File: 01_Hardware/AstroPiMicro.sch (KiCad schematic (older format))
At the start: 40 parts, among them J1 RPi Connector, J10 6-pin JST PH, J2 USB_C_Receptacle_USB2.0, J3 2-pin JST PH, J4 4-pin JST SH, J5 4-pin JST SH, J6 11-pin JST PH, J7 3-pin JST PH, J8 3-pin JST PH, J9 6-pin JST PH, SW1 SW-ON-OFF, U1 LM809, U2 STM32G431KBTx, U3 MCP73831-2-OT, U4 TPS61090, U5 Joystick, Y1 16MHz

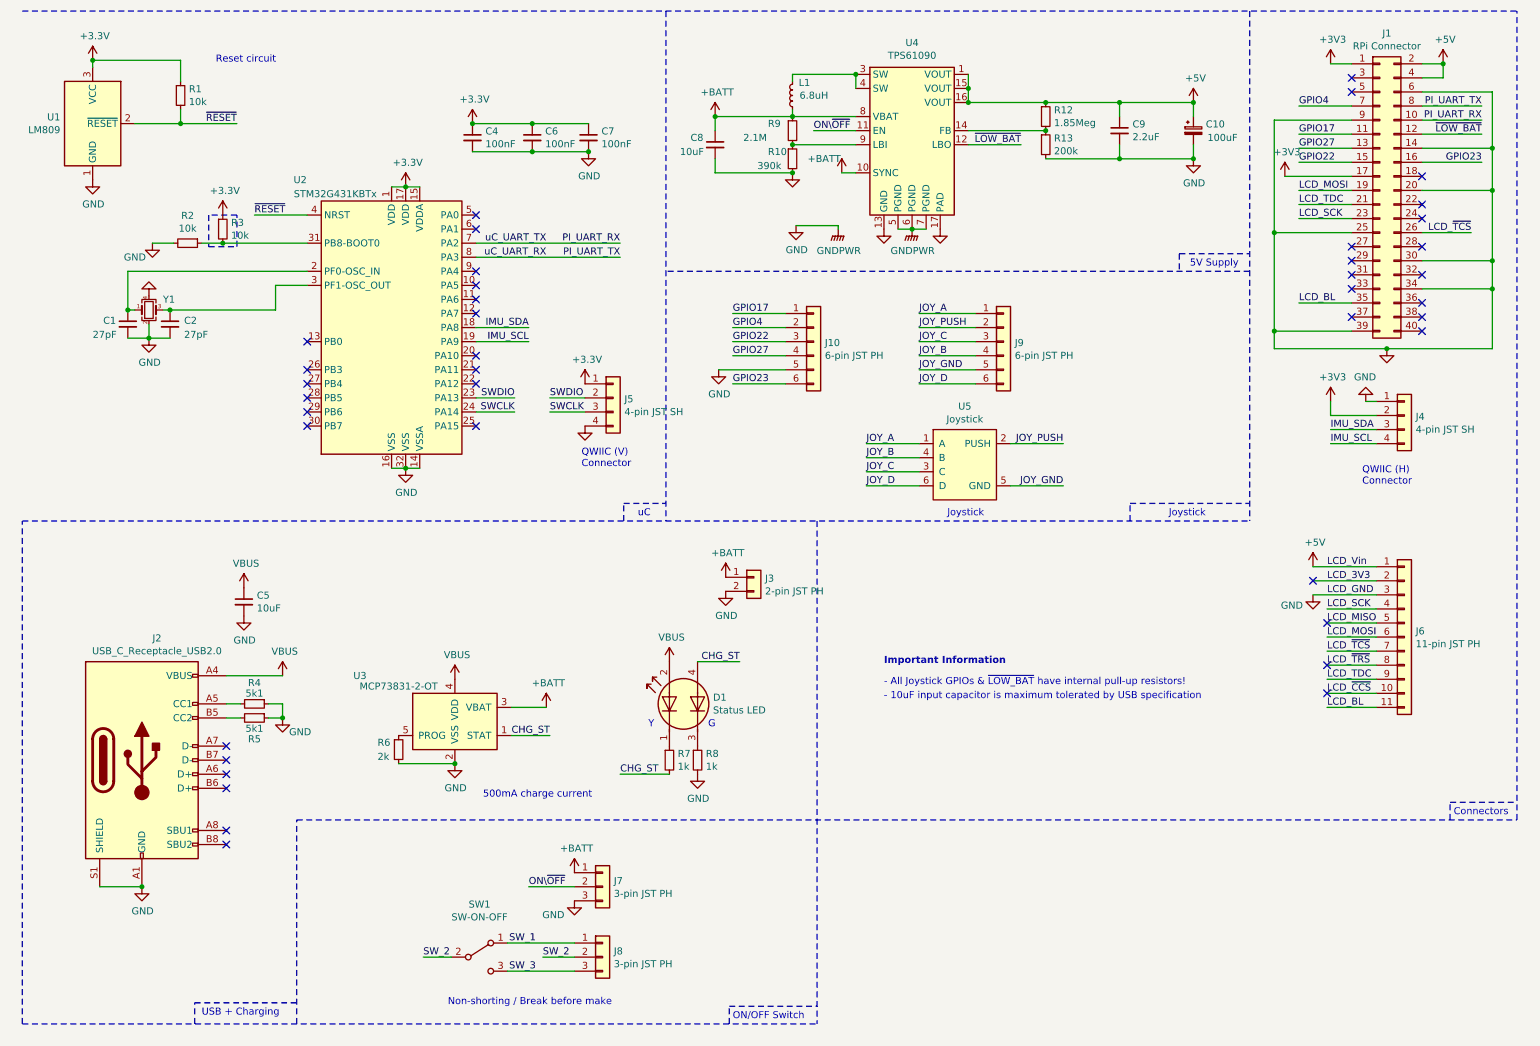
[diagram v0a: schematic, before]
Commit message: Started on HW version 2
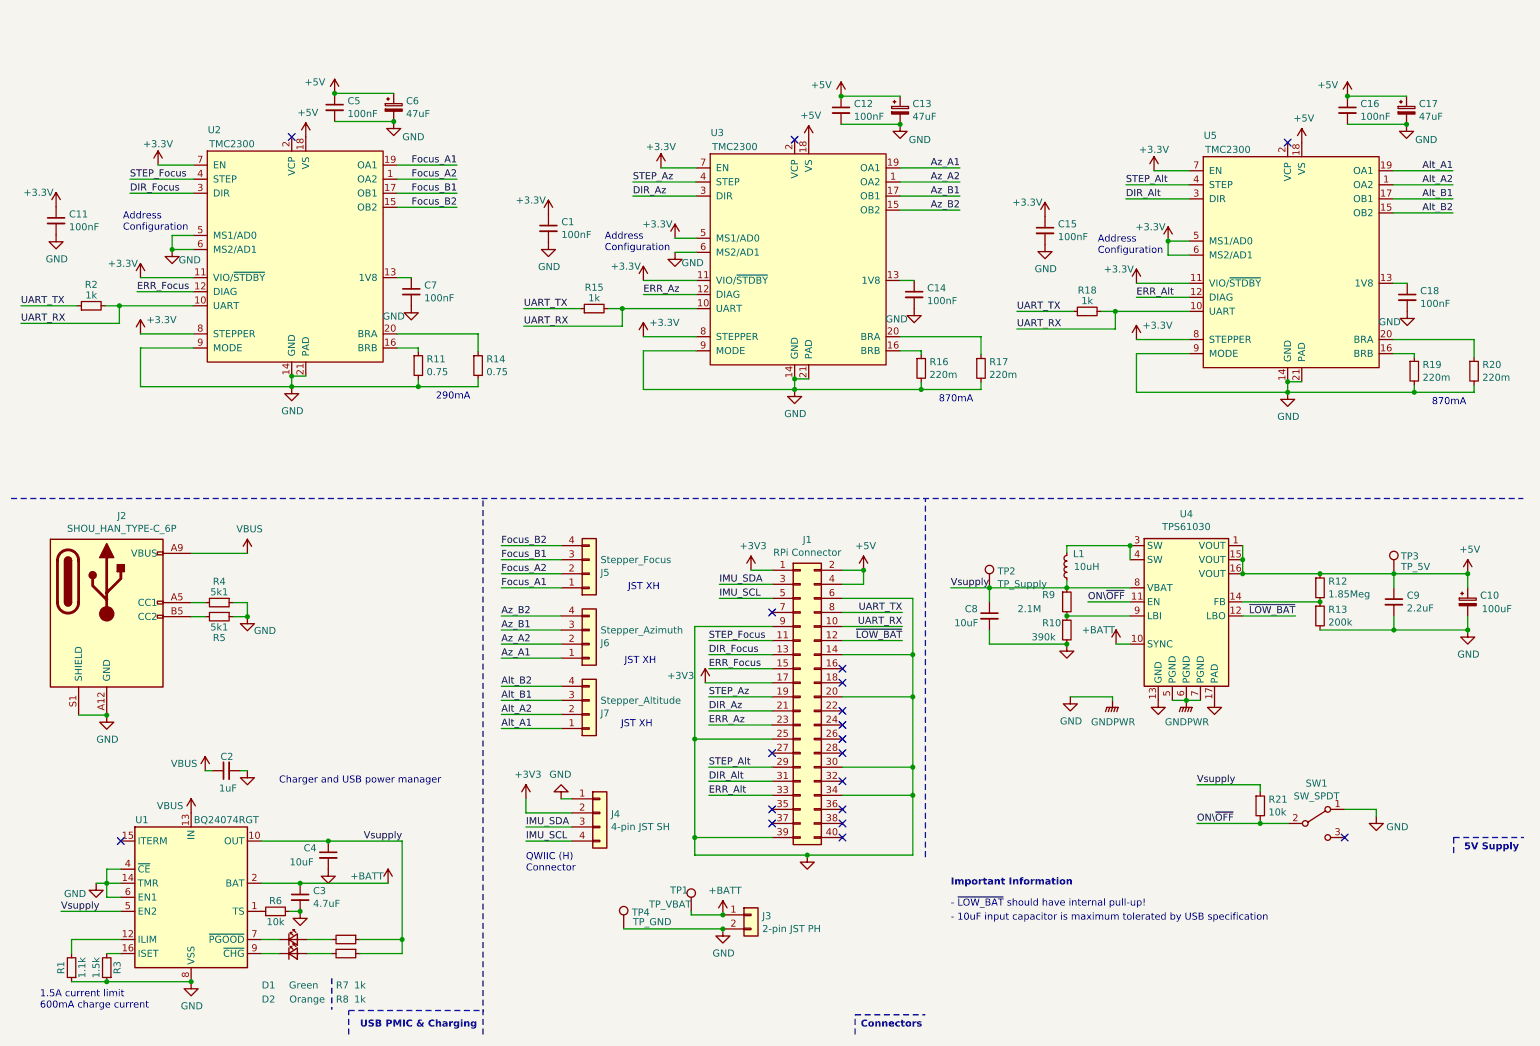
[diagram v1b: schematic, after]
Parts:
- removed C6: 100nF, Capacitor_SMD:C_0603_1608Metric_Pad1.05x0.95mm_HandSolder, symbol Device:C_Small
- removed D1: Status LED, LED_SMD:LED_Avago_PLCC4_3.2x2.8mm_CW, symbol Device:LED_Dual_CACA
- removed J10: 6-pin JST PH, Connector_JST:JST_PH_B6B-PH-K_1x06_P2.00mm_Vertical, symbol Connector_Generic:Conn_01x06
- removed J2: USB_C_Receptacle_USB2.0, astropi:USB_C_GCT_USB4085, symbol Connector:USB_C_Receptacle_USB2.0
- removed J6: 11-pin JST PH, Connector_JST:JST_PH_B11B-PH-K_1x11_P2.00mm_Vertical, symbol Connector_Generic:Conn_01x11
- removed J7: 3-pin JST PH, Connector_JST:JST_PH_B3B-PH-K_1x03_P2.00mm_Vertical, symbol Connector_Generic:Conn_01x03
- removed J8: 3-pin JST PH, Connector_JST:JST_PH_B3B-PH-SM4-TB_1x03-1MP_P2.00mm_Vertical, symbol Connector_Generic:Conn_01x03
- removed J9: 6-pin JST PH, Connector_JST:JST_PH_B6B-PH-SM4-TB_1x06-1MP_P2.00mm_Vertical, symbol Connector_Generic:Conn_01x06
- removed U1: LM809, Package_TO_SOT_SMD:SOT-23, symbol Power_Supervisor:LM809
- removed U2: STM32G431KBTx, Package_QFP:LQFP-32_7x7mm_P0.8mm, symbol MCU_ST_STM32G4:STM32G431KBTx
- removed U3: MCP73831-2-OT, Package_TO_SOT_SMD:SOT-23-5, symbol Battery_Management:MCP73831-2-OT
- removed U5: Joystick, astropi:SKRHAAE010, symbol joystick:SKRHAAE010
- removed Y1: 16MHz, Crystal:Crystal_SMD_Abracon_ABM3B-4Pin_5.0x3.2mm, symbol Device:Crystal_GND24_Small
- added C11, C12, C14, C15, C16, C18: 100nF, Capacitor_SMD:C_0603_1608Metric, symbol Device:C_Small
- added C13, C17, C6: 47uF, Capacitor_Tantalum_SMD:CP_EIA-3528-15_AVX-H, symbol Device:CP_Small
- added C3: 4.7uF, Capacitor_SMD:C_0805_2012Metric, symbol Device:C_Small
- added D1: Green, LED_SMD:LED_0603_1608Metric, symbol Device:LED_Small
- added D2: Orange, LED_SMD:LED_0603_1608Metric, symbol Device:LED_Small
- added J2: SHOU_HAN_TYPE-C_6P, astropi:SHOU HAN TYPE-C 6P, symbol astropi:SHOU_HAN_TYPE-C_6P
- added J6: Stepper_Azimuth, Connector_JST:JST_XH_S4B-XH-A_1x04_P2.50mm_Horizontal, symbol Connector_Generic:Conn_01x04
- added J7: Stepper_Altitude, Connector_JST:JST_XH_S4B-XH-A_1x04_P2.50mm_Horizontal, symbol Connector_Generic:Conn_01x04
- added R11, R14: 0.75, Resistor_SMD:R_0603_1608Metric, symbol Device:R_Small
- added R15, R18: 1k, Resistor_SMD:R_0603_1608Metric, symbol Device:R_Small
- added R16, R17, R19, R20: 220m, Resistor_SMD:R_0603_1608Metric, symbol Device:R_Small
- added R21: 10k, Resistor_SMD:R_0603_1608Metric, symbol Device:R_Small
- added TP1: TP_VBAT, TestPoint:TestPoint_Pad_D2.0mm, symbol Connector:TestPoint
- added TP2: TP_Supply, TestPoint:TestPoint_Pad_D2.0mm, symbol Connector:TestPoint
- added TP3: TP_5V, TestPoint:TestPoint_Pad_D2.0mm, symbol Connector:TestPoint
- added TP4: TP_GND, TestPoint:TestPoint_Pad_2.5x2.5mm, symbol Connector:TestPoint
- added U1: BQ24074RGT, Package_DFN_QFN:VQFN-16-1EP_3x3mm_P0.5mm_EP1.6x1.6mm_ThermalVias, symbol Battery_Management:BQ24074RGT
- added U2, U3, U5: TMC2300, Package_DFN_QFN:QFN-20-1EP_3x3mm_P0.4mm_EP1.65x1.65mm_ThermalVias, symbol astropi:TMC2300
- C1: value 27pF -> 100nF; footprint Capacitor_SMD:C_0603_1608Metric_Pad1.05x0.95mm_HandSolder -> Capacitor_SMD:C_0603_1608Metric; LCSC (none) -> C187860; MPN GRM1885C1H270JA01D -> C0603X104K050T
- C10: footprint Capacitor_Tantalum_SMD:CP_EIA-7343-31_Kemet-D_Pad2.25x2.55mm_HandSolder -> Capacitor_Tantalum_SMD:CP_EIA-7343-15_Kemet-W; LCSC (none) -> C122321
- C2: value 27pF -> 1uF; footprint Capacitor_SMD:C_0603_1608Metric_Pad1.05x0.95mm_HandSolder -> Capacitor_SMD:C_0805_2012Metric; LCSC (none) -> C116352; MPN GRM1885C1H270JA01D -> CL21B105KAFNNNE
- C4: value 100nF -> 10uF; footprint Capacitor_SMD:C_0603_1608Metric_Pad1.05x0.95mm_HandSolder -> Capacitor_SMD:C_0805_2012Metric; LCSC (none) -> C40894; MPN 0603B104K500AT -> 0805X106K250NT
- C5: value 10uF -> 100nF; footprint Capacitor_SMD:C_0805_2012Metric -> Capacitor_SMD:C_0603_1608Metric; LCSC (none) -> C187860; MPN C2012X5R1C106KTJ00E -> C0603X104K050T
- C7: footprint Capacitor_SMD:C_0603_1608Metric_Pad1.05x0.95mm_HandSolder -> Capacitor_SMD:C_0603_1608Metric; LCSC (none) -> C187860; MPN 0603B104K500AT -> C0603X104K050T
- C8: LCSC (none) -> C40894; MPN C2012X5R1C106KTJ00E -> 0805X106K250NT
- C9: LCSC (none) -> C106842
- J3: LCSC (none) -> C47647
- J4: LCSC (none) -> C145956
- J5: value 4-pin JST SH -> Stepper_Focus; footprint Connector_JST:JST_SH_BM04B-SRSS-TB_1x04-1MP_P1.00mm_Vertical -> Connector_JST:JST_XH_S4B-XH-A_1x04_P2.50mm_Horizontal; LCSC (none) -> C157925; MPN A1002WV-S-4P -> S4B-XH-A(LF)(SN)
- L1: value 6.8uH -> 10uH; footprint Inductor_SMD:L_Taiyo-Yuden_NR-50xx_HandSoldering -> astropi:VLS6045EX-100M; LCSC (none) -> C360734; MPN NRS5040T6R8MMGJ -> VLS6045EX-100M
- R1: value 10k -> 1.1k; footprint Resistor_SMD:R_0603_1608Metric_Pad1.05x0.95mm_HandSolder -> Resistor_SMD:R_0603_1608Metric; LCSC (none) -> C22764; MPN 0603WAJ0103T5E -> 0603WAF1101T5E
- R10: footprint Resistor_SMD:R_0603_1608Metric_Pad1.05x0.95mm_HandSolder -> Resistor_SMD:R_0603_1608Metric; LCSC (none) -> C307295
- R12: footprint Resistor_SMD:R_0603_1608Metric_Pad1.05x0.95mm_HandSolder -> Resistor_SMD:R_0603_1608Metric; LCSC (none) -> C61679
- R13: footprint Resistor_SMD:R_0603_1608Metric_Pad1.05x0.95mm_HandSolder -> Resistor_SMD:R_0603_1608Metric; LCSC (none) -> C22949
- R2: value 10k -> 1k; footprint Resistor_SMD:R_0603_1608Metric_Pad1.05x0.95mm_HandSolder -> Resistor_SMD:R_0603_1608Metric; LCSC (none) -> C101253; MPN 0603WAJ0103T5E -> CR0603JA0102G
- R3: value 10k -> 1.5k; footprint Resistor_SMD:R_0603_1608Metric_Pad1.05x0.95mm_HandSolder -> Resistor_SMD:R_0603_1608Metric; LCSC (none) -> C114680; MPN 0603WAJ0103T5E -> RC0603JR-071K5L
- R4, R5: footprint Resistor_SMD:R_0603_1608Metric_Pad1.05x0.95mm_HandSolder -> Resistor_SMD:R_0603_1608Metric; LCSC (none) -> C23186
- R6: value 2k -> 10k; footprint Resistor_SMD:R_0603_1608Metric_Pad1.05x0.95mm_HandSolder -> Resistor_SMD:R_0603_1608Metric; LCSC (none) -> C99198; MPN CR0603FA2001G -> RC0603JR-0710KL
- R7, R8: footprint Resistor_SMD:R_0603_1608Metric_Pad1.05x0.95mm_HandSolder -> Resistor_SMD:R_0603_1608Metric; LCSC (none) -> C101253; MPN 0603WAF1001T5E -> CR0603JA0102G
- R9: footprint Resistor_SMD:R_0603_1608Metric_Pad1.05x0.95mm_HandSolder -> Resistor_SMD:R_0603_1608Metric; LCSC (none) -> C166860
- SW1: value SW-ON-OFF -> SW_SPDT; footprint astropi:SSSS213202 -> Button_Switch_SMD:SW_SPDT_CK-JS102011SAQN; LCSC (none) -> C221660; MPN SSSS213202 -> JS102011SAQN
- U4: value TPS61090 -> TPS61030; LCSC (none) -> C10110; MPN TPS61090RSAR -> TPS61030RSAR
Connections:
- net SW_1 is gone; now on net GND: SW1.1 (A)
- net SW_2 is gone; now on net ON\~OFF: SW1.2 (B)
- net +3V3: now also C1.1, C11.1, C15.1, U2.11 (VIO/~STDBY), U2.7 (EN), U2.8 (STEPPER), U3.11 (VIO/~STDBY), U3.5 (MS1/AD0), U3.7 (EN), U3.8 (STEPPER), U5.11 (VIO/~STDBY), U5.5 (MS1/AD0), U5.6 (MS2/AD1), U5.7 (EN), U5.8 (STEPPER); no longer C4.1, C7.1, J5.1 (Pin_1), R1.1, R3.1
- net +5V: now also C5.1, C12.1, C13.1, C16.1, C17.1, C6.1, TP3.1, U2.18 (VS), U3.18 (VS), U5.18 (VS)
- net +BATT: now also C3.1, TP1.1, U1.2 (BAT), U1.3 (BAT); no longer C8.1, L1.1, R9.1, U4.8 (VBAT)
- net GND: now also R1.1, R3.1, C11.2, C12.2, C13.2, C14.2, C15.2, C16.2, C17.2, C18.2, C3.2, C6.2, J2.A12 (GND), J2.B12 (GND), J2.S1 (SHIELD), R11.2, R14.2, R16.2, R17.2, R19.2, R20.2, TP4.1, U1.14 (TMR), U1.17 (VSS), U1.4 (~CE), U1.6 (EN1), U1.8 (VSS), U2.14 (GND), U2.21 (PAD), U2.5 (MS1/AD0), U2.6 (MS2/AD1), U2.9 (MODE), U3.14 (GND), U3.21 (PAD), U3.6 (MS2/AD1), U3.9 (MODE), U5.14 (GND), U5.21 (PAD), U5.9 (MODE); no longer J5.4 (Pin_4), R2.2, R8.2
- net IMU_SCL: now also J1.5 (Pin_5)
- net IMU_SDA: now also J1.3 (Pin_3)
- net ON\~OFF: now also R21.2
- net VBUS: now also C2.1, J2.A9 (VBUS), J2.B9 (VBUS), U1.13 (IN); no longer C5.1
- net STEP_Alt: now reaches J1.29 (Pin_29)
- net STEP_Alt: now also U5.4 (STEP)
- net DIR_Alt: now reaches J1.31 (Pin_31)
- net DIR_Alt: now also U5.3 (DIR)
- net ERR_Alt: now reaches J1.33 (Pin_33)
- net ERR_Alt: now also U5.12 (DIAG)
- net at R4.2: now also J2.A5 (CC1)
- net at R5.2: now also J2.B5 (CC2)
- net Vsupply: now reaches R7.1
- net Vsupply: now also C4.1, C8.1, L1.1, R8.1, R9.1, U4.8 (VBAT), R21.1, TP2.1, U1.10 (OUT), U1.11 (OUT), U1.5 (EN2)
- net at R6.1: now also U1.1 (TS)
- net at R3.2: now also U1.16 (ISET); no longer R2.1
- net CHG_ST: no longer names the net of R7.2
- net CHG_ST: now also D1.2 (A)
- net GPIO17 renamed STEP_Focus
- net STEP_Focus: now also U2.4 (STEP)
- net GPIO22 renamed ERR_Focus
- net ERR_Focus: now also U2.12 (DIAG)
- net GPIO23: no longer names the net of J1.16 (Pin_16)
- net GPIO27 renamed DIR_Focus
- net DIR_Focus: now also U2.3 (DIR)
- net GPIO4: no longer names the net of J1.7 (Pin_7)
- net LCD_BL: no longer names the net of J1.35 (Pin_35)
- net LCD_MOSI renamed STEP_Az
- net STEP_Az: now also U3.4 (STEP)
- net LCD_SCK renamed ERR_Az
- net ERR_Az: now also U3.12 (DIAG)
- net LCD_TDC renamed DIR_Az
- net DIR_Az: now also U3.3 (DIR)
- net LCD_~TCS: no longer names the net of J1.26 (Pin_26)
- net PI_UART_RX renamed UART_RX
- net UART_RX: now also R2.2, R15.2, R18.2, U2.10 (UART), U3.10 (UART), U5.10 (UART)
- net PI_UART_TX renamed UART_TX
- net UART_TX: now also R2.1, R15.1, R18.1
- net SWCLK renamed Focus_B1
- net Focus_B1: now also U2.17 (OB1)
- net SWDIO renamed Focus_A2
- net Focus_A2: now also U2.1 (OA2)
- net SW_3: no longer names the net of SW1.3 (C)
- net ~RESET: no longer names the net of R1.2
- net ~RESET: now also U1.12 (ILIM)
- new net: C7.1, U2.13 (1V8)
- new net: R11.1, U2.16 (BRB)
- new net: R14.1, U2.20 (BRA)
- new net: C14.1, U3.13 (1V8)
- new net: R16.1, U3.16 (BRB)
- new net: R17.1, U3.20 (BRA)
- new net: C18.1, U5.13 (1V8)
- new net: R19.1, U5.16 (BRB)
- new net: R20.1, U5.20 (BRA)
- new net: D1.1 (K), U1.7 (~PGOOD)
- new net: D2.1 (K), U1.9 (~CHG)
- new net: D2.2 (A), R8.2
- new net Alt_A1: J7.1 (Pin_1), U5.19 (OA1)
- new net Alt_A2: J7.2 (Pin_2), U5.1 (OA2)
- new net Alt_B1: J7.3 (Pin_3), U5.17 (OB1)
- new net Alt_B2: J7.4 (Pin_4), U5.15 (OB2)
- new net Az_A1: J6.1 (Pin_1), U3.19 (OA1)
- new net Az_A2: J6.2 (Pin_2), U3.1 (OA2)
- new net Az_B1: J6.3 (Pin_3), U3.17 (OB1)
- new net Az_B2: J6.4 (Pin_4), U3.15 (OB2)
- new net Focus_A1: J5.1 (Pin_1), U2.19 (OA1)
- new net Focus_B2: J5.4 (Pin_4), U2.15 (OB2)
- no-connect marks 41 -> 19
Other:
- note added: "- ~LOW_BAT~ should have internal pull-up!"
- note added: "1.5A current limit\n600mA charge current"
- note added: "290mA"
- note added: "870mA"
- note added: "Address\nConfiguration"
- note added: "Charger and USB power manager"
- note added: "JST XH"
- note added: "USB PMIC & Charging"
- note removed: "- All Joystick GPIOs & ~LOW_BAT~ have internal pull-up resistors!"
- note removed: "500mA charge current"
- note removed: "G"
- note removed: "Joystick"
- note removed: "Non-shorting / Break before make"
- note removed: "ON/OFF Switch"
- note removed: "QWIIC (V)\nConnector"
- note removed: "Reset circuit"
- note removed: "USB + Charging"
- note removed: "Y"
- note removed: "uC"
- moved on the sheet: C10, C8, C9, J1, J3, J4, L1, R10, R12, R13, R4, R5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
